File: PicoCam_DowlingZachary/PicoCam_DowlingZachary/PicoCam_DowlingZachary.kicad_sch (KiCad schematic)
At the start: 58 parts, among them J1 USB4105-GF-A, J2 LEFT, J3 DEBUG, J4 RIGHT, Q1 FDG6320C, SW1 PCM12, SW2 SW_MEC_5G, U1 W25Q128JV, U2 RP2040, U3 MCP1702T-3302E_CB, U4 MCP73831T-2ACI_OT, U5 TPS2113APW, Y1 12MHz

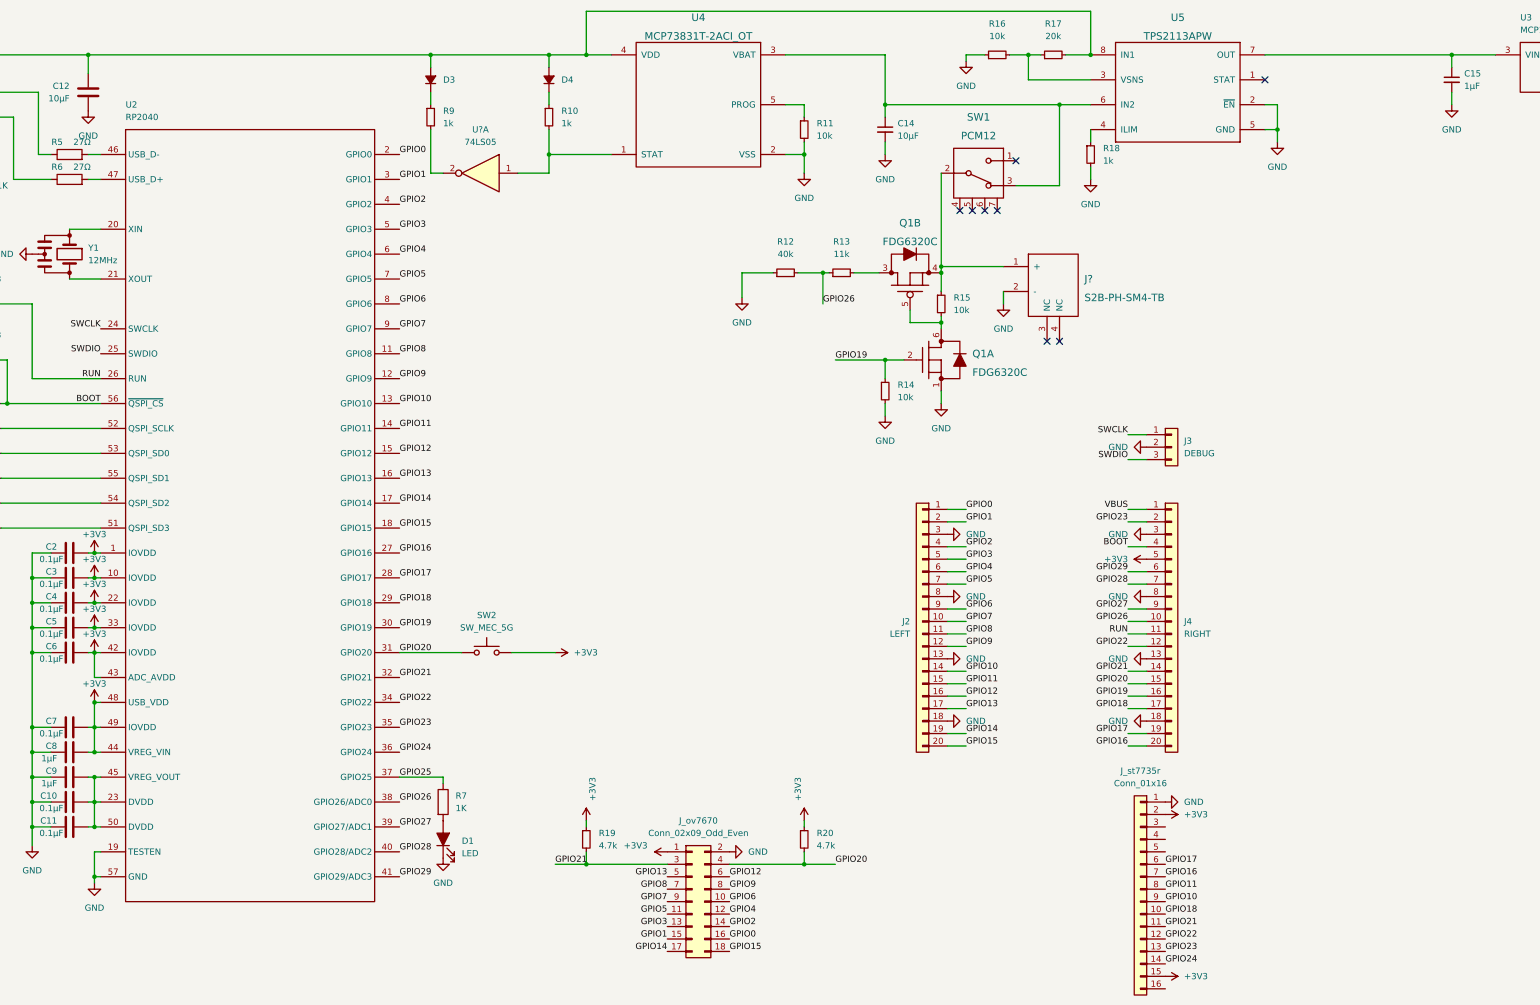
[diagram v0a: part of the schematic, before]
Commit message: update
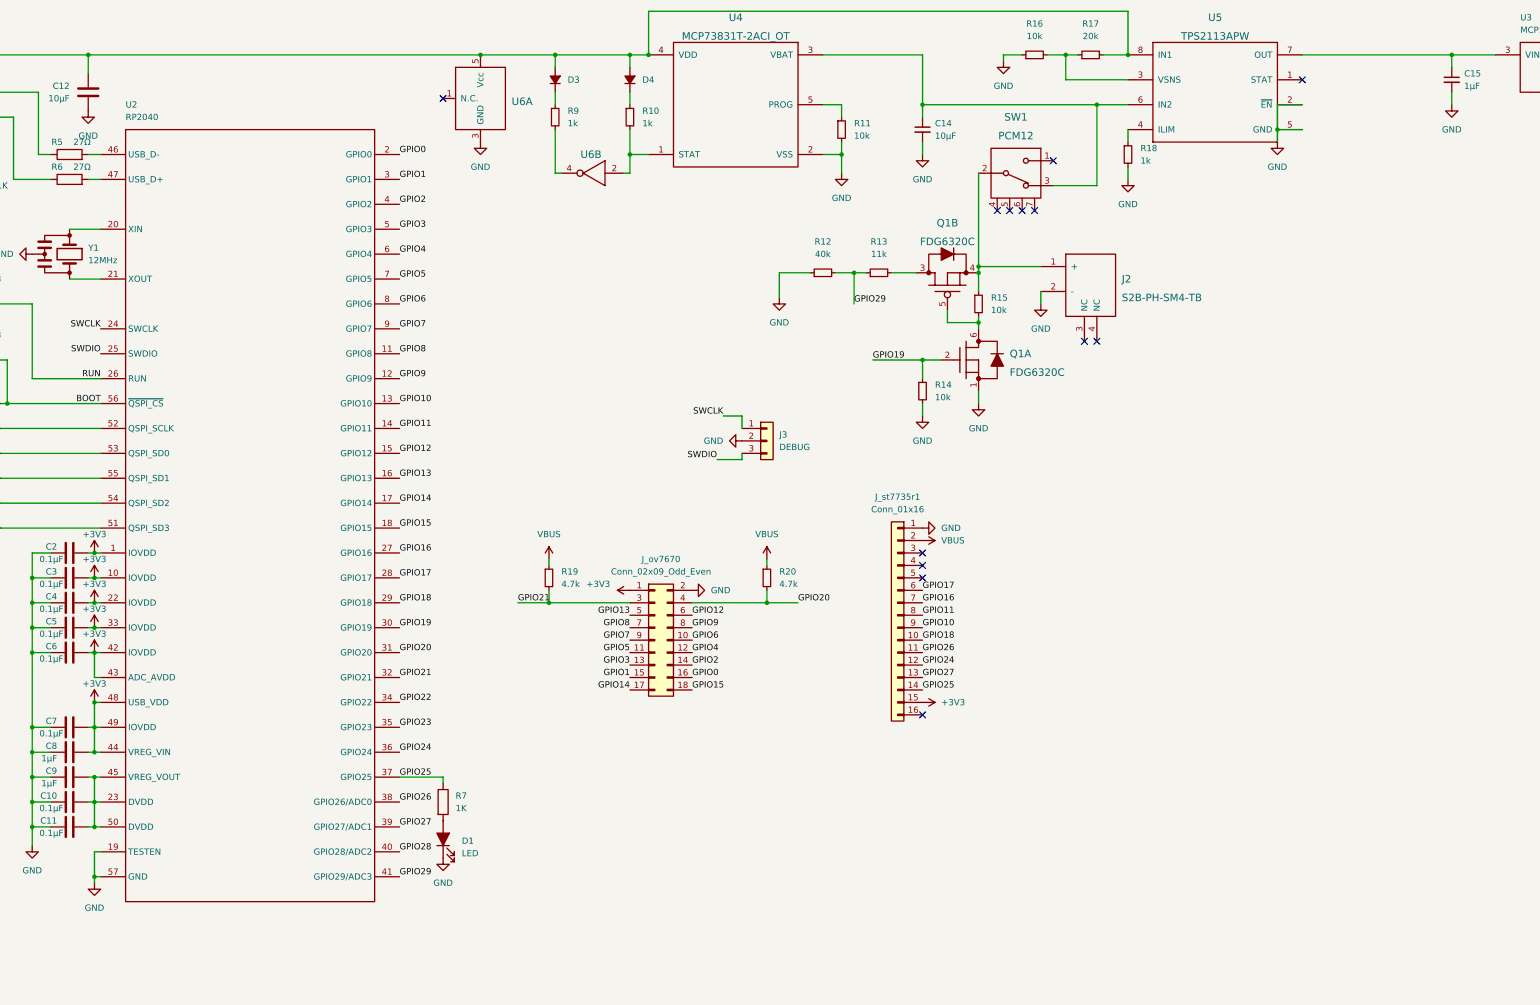
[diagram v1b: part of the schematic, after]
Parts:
- removed J2: LEFT, symbol Connector_Generic:Conn_01x20
- removed J4: RIGHT, symbol Connector_Generic:Conn_01x20
- removed SW2: SW_MEC_5G, symbol Switch:SW_MEC_5G
- removed U?: 74LS05, symbol 74xx:74LS05
- added U6: SN74LVC1GU04, Package_TO_SOT_SMD:SOT-353_SC-70-5, symbol Eclectronics:SN74LVC1GU04
- C1, C10, C11, C15, C2, C3, C4, C5, C6, C7, C8, C9: footprint (none) -> Capacitor_SMD:C_0402_1005Metric
- C12, C13, C14: footprint (none) -> Capacitor_SMD:C_0603_1608Metric
- D1, D2, D3, D4: footprint (none) -> LED_SMD:LED_0805_2012Metric
- J1: footprint (none) -> Eclectronics:USB4105-GF-A
- J2: renamed from J?; footprint (none) -> Eclectronics:JST_S2B-PH-SM4-TB(LF)(SN)
- J3: footprint (none) -> Connector_PinHeader_2.54mm:PinHeader_1x03_P2.54mm_Vertical
- J_ov7670: footprint (none) -> Connector_PinHeader_2.54mm:PinHeader_2x09_P2.54mm_Vertical
- J_st7735r1: renamed from J_st7735r; footprint (none) -> Connector_PinHeader_2.54mm:PinHeader_1x16_P2.54mm_Vertical
- Q1: footprint (none) -> Package_TO_SOT_SMD:SOT-363_SC-70-6
- R1, R10, R18, R2, R3, R4, R5, R6, R7, R8, R9: footprint (none) -> Resistor_SMD:R_0402_1005Metric
- R11, R12, R13, R14, R15, R16, R17, R19, R20: footprint (none) -> Resistor_SMD:R_0603_1608Metric
- S1, S2: footprint (none) -> Eclectronics:KXT321LHS
- SW1: footprint (none) -> Eclectronics:SW_PCM12SMTR
- U1: footprint (none) -> Eclectronics:MIC_WSON-8
- U2: footprint (none) -> Eclectronics:RP2040
- U3: footprint (none) -> Package_TO_SOT_SMD:SOT-23
- U4: footprint (none) -> Package_TO_SOT_SMD:SOT-23-5
- U5: footprint (none) -> Package_SO:TSSOP-8_4.4x3mm_P0.65mm
- Y1: footprint (none) -> Eclectronics:CSTNE
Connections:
- net +3V3: no longer J_st7735r1.2 (Pin_2), R19.1, R20.1
- net GND: now also U6.3 (GND)
- net GPIO21: no longer J_st7735r1.11 (Pin_11)
- net GPIO22: no longer J_st7735r1.12 (Pin_12)
- net GPIO23: no longer J_st7735r1.13 (Pin_13)
- net GPIO24: now also J_st7735r1.12 (Pin_12); no longer J_st7735r1.14 (Pin_14)
- net GPIO25: now also J_st7735r1.14 (Pin_14)
- net GPIO26: now also J_st7735r1.11 (Pin_11); no longer R12.2, R13.1
- net GPIO27: now also J_st7735r1.13 (Pin_13)
- net GPIO29: now also R12.2, R13.1
- net VBUS: now also J_st7735r1.2 (Pin_2), R19.1, R20.1, U6.5 (Vcc)
- net at R10.2, U4.1 (STAT): now also U6.2
- net at R9.2: now also U6.4
- no-connect marks 10 -> 15
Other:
- moved on the sheet: C14, D3, D4, J2, J3, J_ov7670, J_st7735r1, Q1A, Q1B, R10, R11, R12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

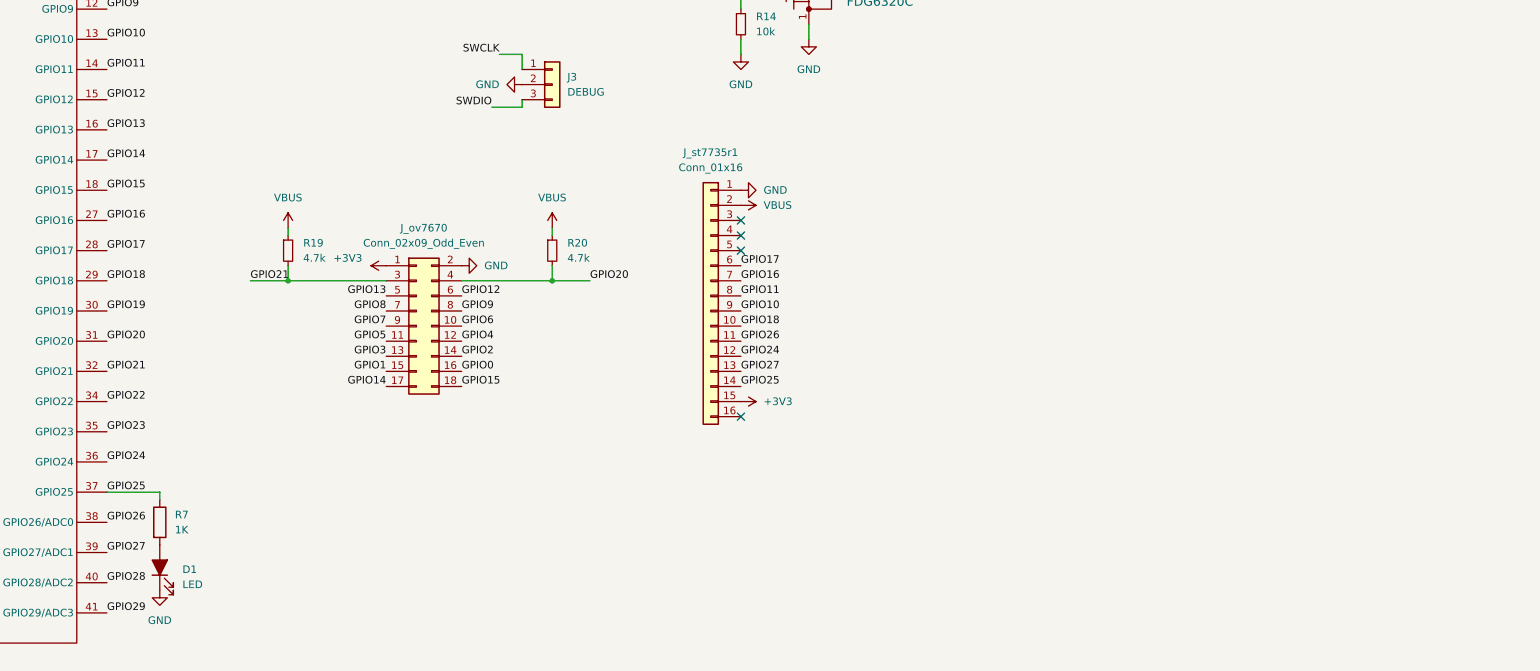
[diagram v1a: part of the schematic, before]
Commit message: button
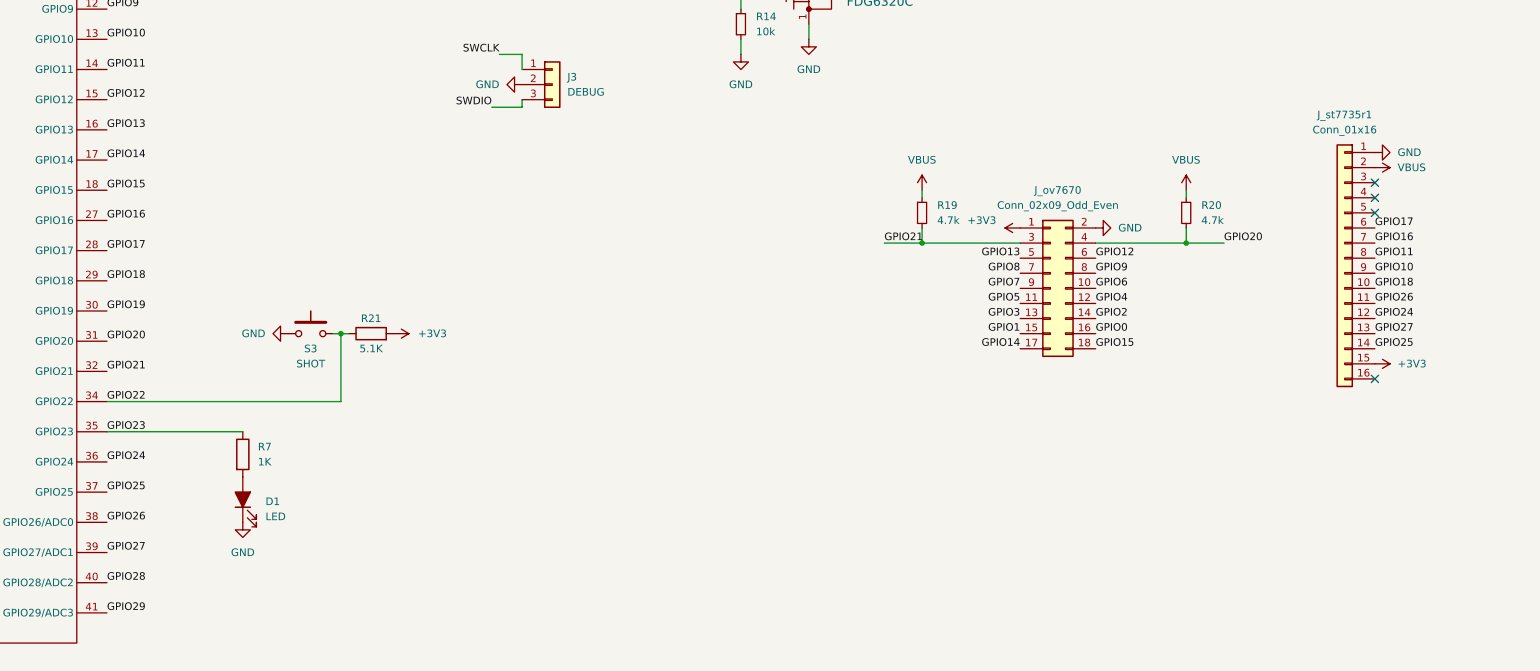
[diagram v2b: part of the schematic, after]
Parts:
- added R21: 5.1K, Resistor_SMD:R_0402_1005Metric, symbol Device:R
- added S3: SHOT, Eclectronics:KXT321LHS, symbol Eclectronics:SW
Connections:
- net +3V3: now also R21.2
- net GND: now also S3.1
- net GPIO22: now also R21.1, S3.2
- net GPIO23: now also R7.1
- net GPIO25: no longer R7.1
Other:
- moved on the sheet: D1, J_ov7670, J_st7735r1, R19, R20, R7

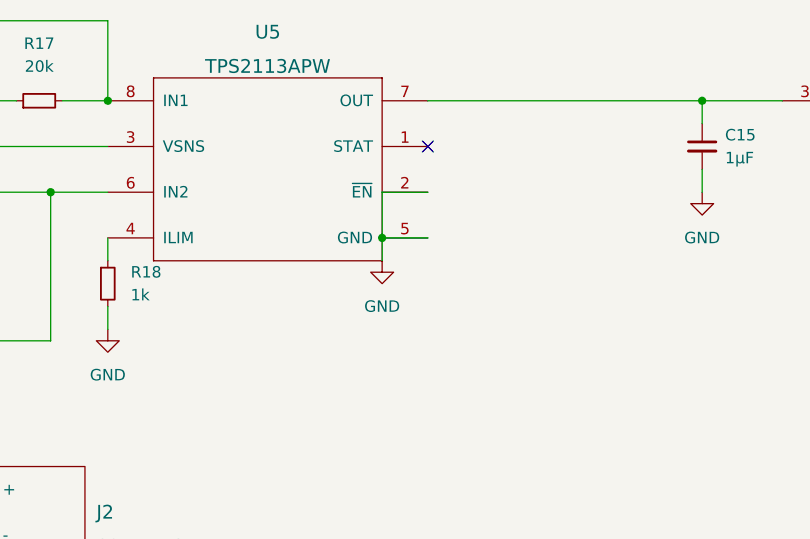
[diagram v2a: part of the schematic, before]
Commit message: update
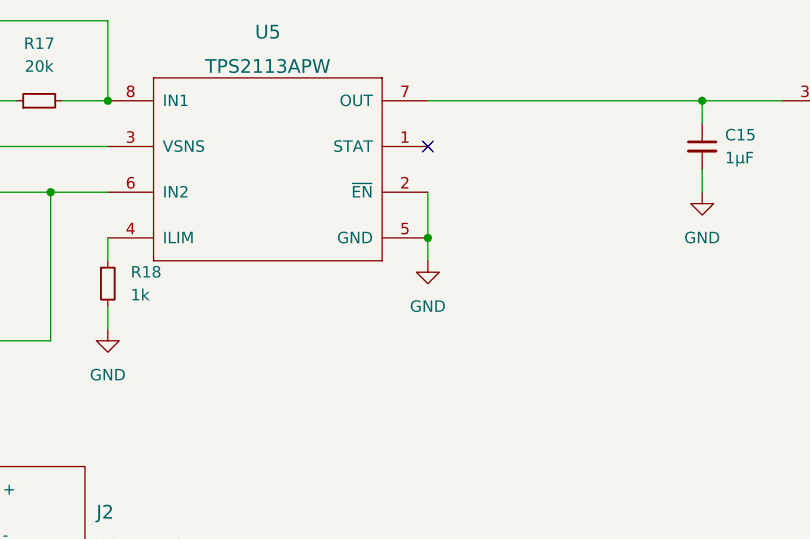
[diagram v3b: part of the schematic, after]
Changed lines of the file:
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@@
   (junction (at 290.83 24.13) (diameter 0) (color 0 0 0 0)
   )
+  (junction (at 326.39 39.37) (diameter 0) (color 0 0 0 0)
+  )
   (junction (at 260.35 78.74) (diameter 0) (color 0 0 0 0)
   )
@@
   )
   (junction (at 67.31 181.61) (diameter 0) (color 0 0 0 0)
-  )
-  (junction (at 321.31 39.37) (diameter 0) (color 0 0 0 0)
   )
   (junction (at 24.13 62.23) (diameter 0) (color 0 0 0 0)
@@
     (stroke (width 0) (type default) (color 0 0 0 0))
   )
+  (wire (pts (xy 326.39 34.29) (xy 326.39 39.37))
+    (stroke (width 0) (type default) (color 0 0 0 0))
+  )
   (wire (pts (xy 67.31 161.29) (xy 71.12 161.29))
     (stroke (width 0) (type default) (color 0 0 0 0))
@@
     (stroke (width 0) (type default) (color 0 0 0 0))
   )
-  (wire (pts (xy 321.31 39.37) (xy 321.31 41.91))
+  (wire (pts (xy 326.39 39.37) (xy 326.39 41.91))
     (stroke (width 0) (type default) (color 0 0 0 0))
   )
@@
     (stroke (width 0) (type default) (color 0 0 0 0))
   )
-  (wire (pts (xy 326.39 34.29) (xy 321.31 34.29))
-    (stroke (width 0) (type default) (color 0 0 0 0))
-  )
   (wire (pts (xy 41.91 26.67) (xy 40.64 26.67))
     (stroke (width 0) (type default) (color 0 0 0 0))
@@
     (stroke (width 0) (type default) (color 0 0 0 0))
   )
-  (wire (pts (xy 326.39 39.37) (xy 321.31 39.37))
-    (stroke (width 0) (type default) (color 0 0 0 0))
-  )
   (wire (pts (xy 41.91 24.13) (xy 78.74 24.13))
     (stroke (width 0) (type default) (color 0 0 0 0))
@@
   )
   (wire (pts (xy 234.95 68.58) (xy 234.95 74.93))
-    (stroke (width 0) (type default) (color 0 0 0 0))
-  )
-  (wire (pts (xy 321.31 34.29) (xy 321.31 39.37))
     (stroke (width 0) (type default) (color 0 0 0 0))
   )
@@
     (pin "3")
   )
-  (symbol (lib_id "power:GND") (at 321.31 41.91 0) (unit 1)
+  (symbol (lib_id "power:GND") (at 326.39 41.91 0) (unit 1)
     (in_bom yes) (on_board yes) (fields_autoplaced)
-    (property "Reference" "#PWR0102" (id 0) (at 321.31 48.26 0)
+    (property "Reference" "#PWR0102" (id 0) (at 326.39 48.26 0)
       (effects (font (size 1.27 1.27)) hide)
     )
-    (property "Value" "GND" (id 1) (at 321.31 46.99 0))
-    (property "Footprint" "" (id 2) (at 321.31 41.91 0)
+    (property "Value" "GND" (id 1) (at 326.39 46.99 0))
+    (property "Footprint" "" (id 2) (at 326.39 41.91 0)
       (effects (font (size 1.27 1.27)) hide)
     )
-    (property "Datasheet" "" (id 3) (at 321.31 41.91 0)
+    (property "Datasheet" "" (id 3) (at 326.39 41.91 0)
       (effects (font (size 1.27 1.27)) hide)
     )
